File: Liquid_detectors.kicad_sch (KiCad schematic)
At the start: 1 part, among them U1 AD8021AR

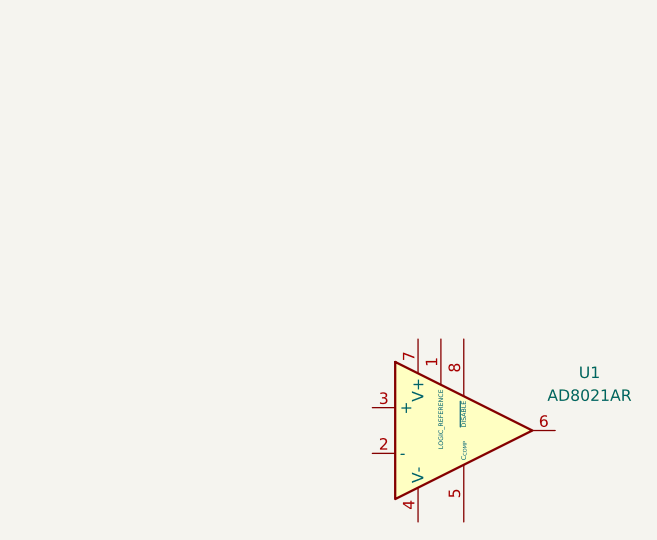
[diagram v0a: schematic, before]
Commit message: ahora modifique dos sch
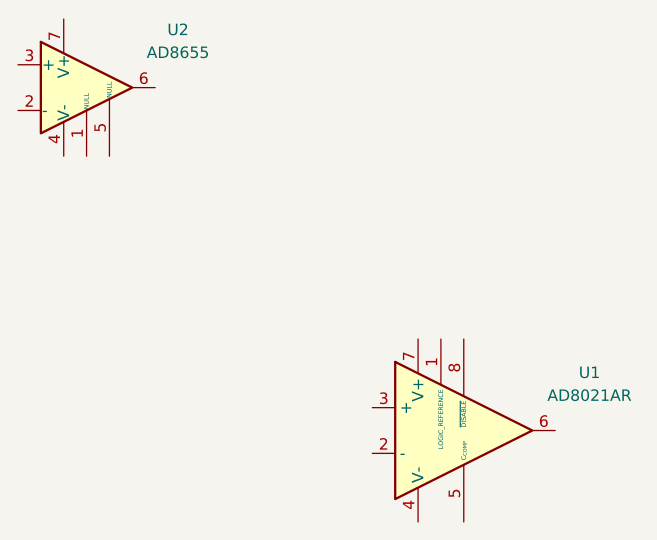
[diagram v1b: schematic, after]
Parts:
- added U2: AD8655, symbol Amplifier_Operational:AD8655
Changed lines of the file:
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@@
+		)
+	)
+	(symbol
+		(lib_id "Amplifier_Operational:AD8655")
+		(at 113.03 53.34 0)
+		(unit 1)
+		(exclude_from_sim no)
+		(in_bom yes)
+		(on_board yes)
+		(dnp no)
+		(fields_autoplaced yes)
+		(property "Reference" "U2"
+			(at 123.19 46.9198 0)
+			(effects
+				(font
+					(size 1.27 1.27)
+				)
+			)
+		)
+		(property "Value" "AD8655"
+			(at 123.19 49.4598 0)
+			(effects
+				(font
+					(size 1.27 1.27)
+				)
+			)
+		)
+		(property "Footprint" ""
+			(at 114.3 52.07 0)
+			(effects
+				(font
+					(size 1.27 1.27)
+				)
+				(hide yes)
+			)
+		)
+		(property "Datasheet" "https://www.analog.com/media/en/technical-documentation/data-sheets/ad8655_8656.pdf"
+			(at 116.84 49.53 0)
+			(effects
+				(font
+					(size 1.27 1.27)
+				)
+				(hide yes)
+			)
+		)
+		(property "Description" "Single Low Noise, Precision CMOS Amplifier"
+			(at 113.03 53.34 0)
+			(effects
+				(font
+					(size 1.27 1.27)
+				)
+				(hide yes)
+			)
+		)
+		(pin "3"
+		)
+		(pin "2"
+		)
+		(pin "7"
+		)
+		(pin "4"
+		)
+		(pin "8"
+		)
+		(pin "1"
+		)
+		(pin "5"
+		)
+		(pin "6"
+		)
+		(instances
+			(project ""
+				(path "/e23e72d0-3a4b-405e-bd06-0639cdab408e"
+					(reference "U2")
+					(unit 1)
+				)
+			)
 		)
 	)
